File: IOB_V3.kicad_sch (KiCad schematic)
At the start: 6 parts, among them J1 Conn_01x02, J2 Conn_01x03, U1 REF3033

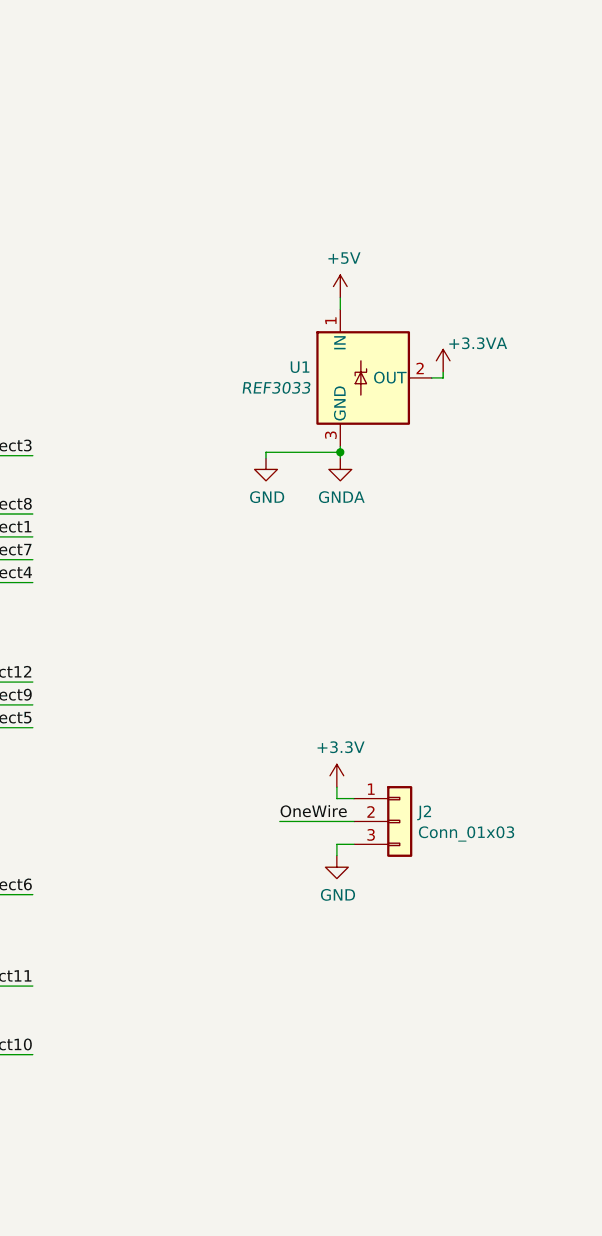
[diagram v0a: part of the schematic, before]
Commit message: WIP
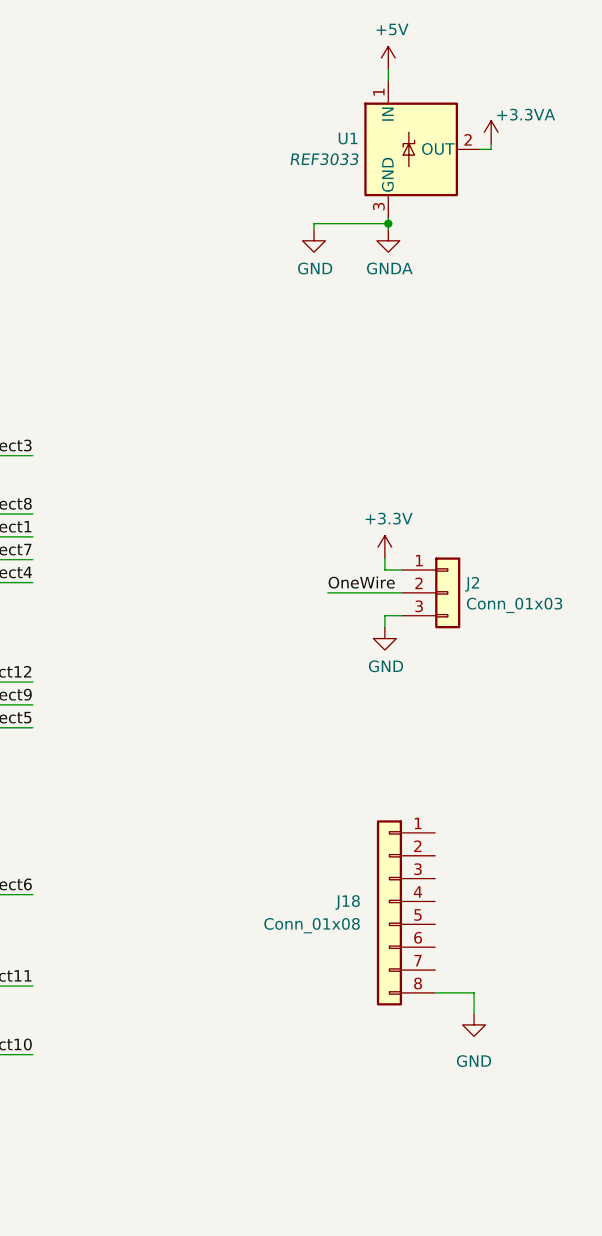
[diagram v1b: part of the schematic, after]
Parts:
- added J18: Conn_01x08, Connector_IDC:IDC-Header_2x04_P2.54mm_Horizontal, symbol Connector_Generic:Conn_01x08
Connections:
- net GND: now also J18.8 (Pin_8)
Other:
- moved on the sheet: J2, U1
